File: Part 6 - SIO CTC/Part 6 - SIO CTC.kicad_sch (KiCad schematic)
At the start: 33 parts, among them J1 EDGE, J2 USB B, J3 DB9-F, J4 EXT LCD, U1 Z84C4010, U2 MCP2221A, U3 74AC138, U4 MAX232, U5 Z84C3010, U6 Z84C4010, U7 74HC563

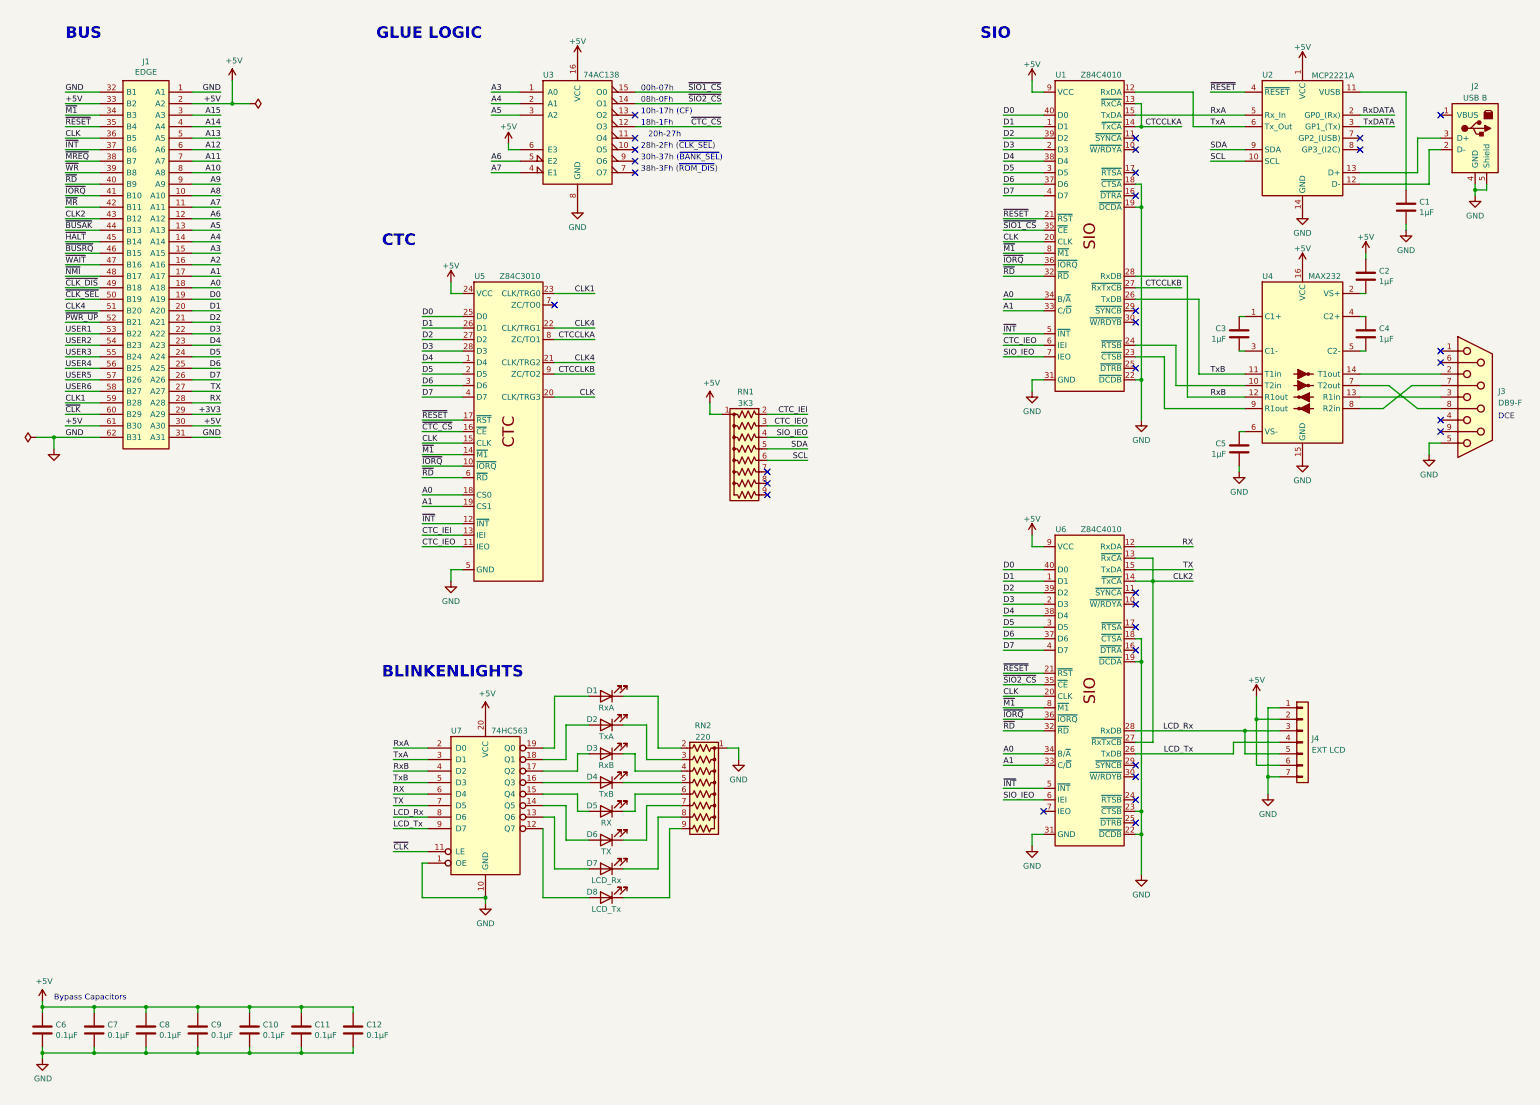
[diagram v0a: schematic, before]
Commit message: Long time backup
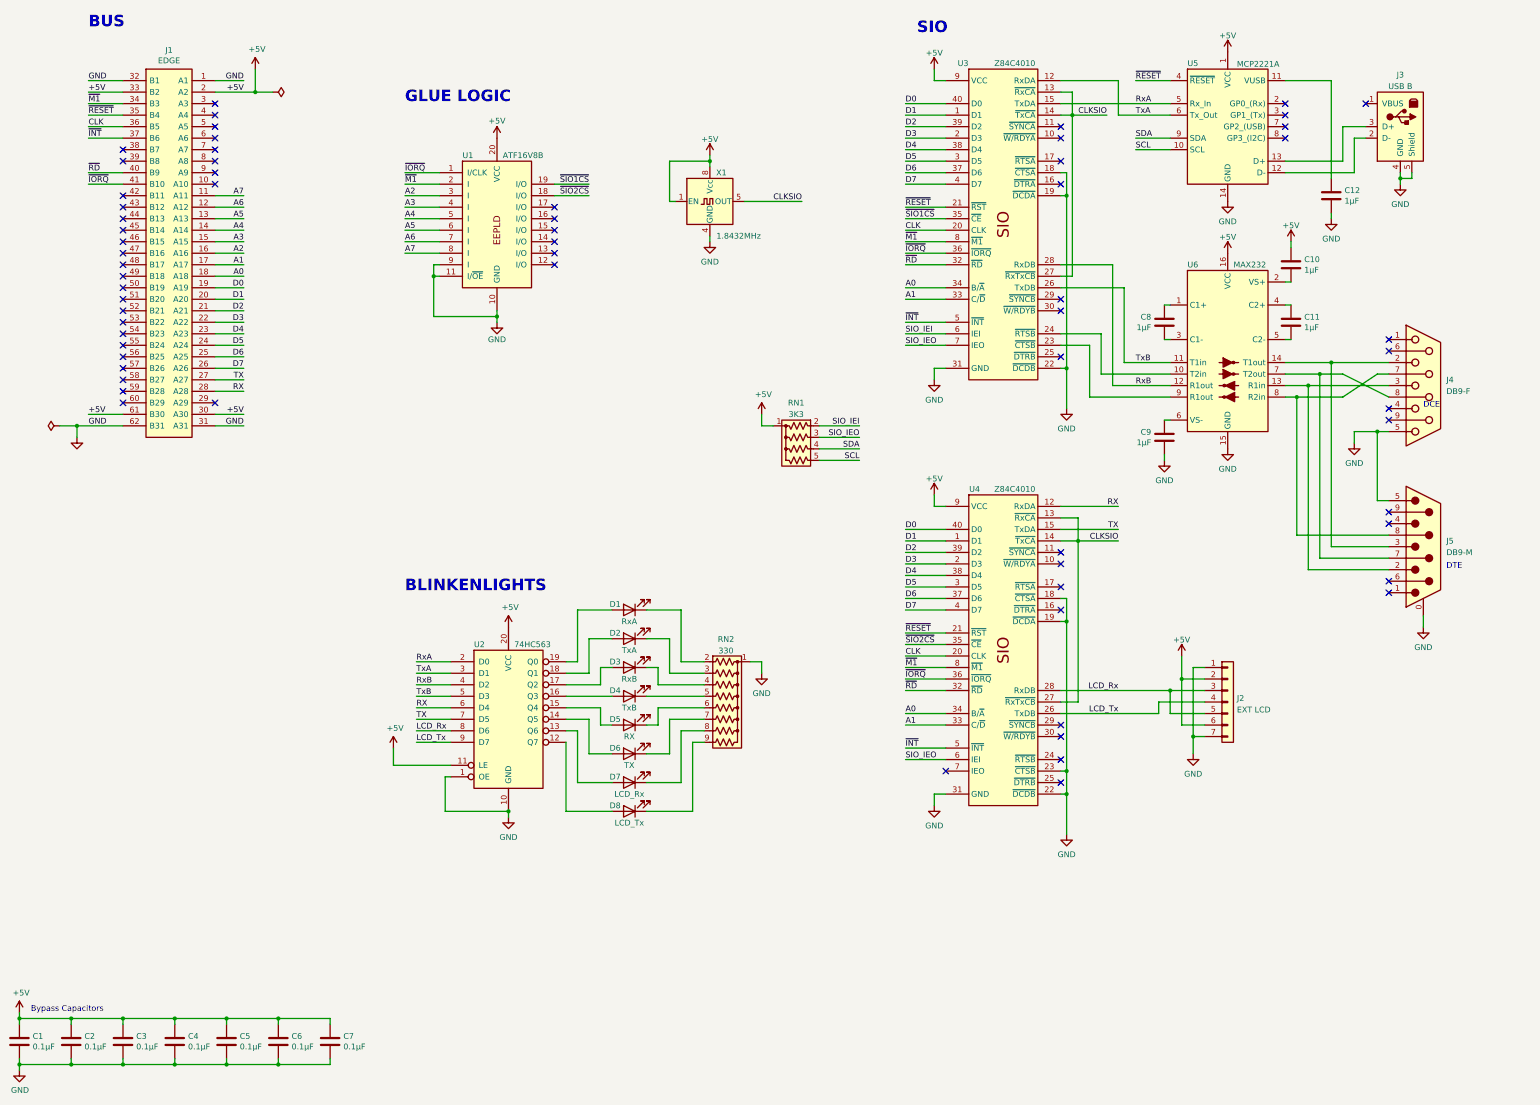
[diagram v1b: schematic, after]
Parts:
- removed RN1: 3K3, Resistor_THT:R_Array_SIP9, symbol Device:R_Network08_US
- removed U3: 74AC138, Package_DIP:DIP-16_W7.62mm_Socket, symbol 74xx:74LS138
- removed U5: Z84C3010, Package_DIP:DIP-28_W15.24mm_Socket, symbol 0_Z80_Library:Z84C30xx CTC
- added J5: DB9-M, Connector_Dsub:DSUB-9_Male_Horizontal_P2.77x2.84mm_EdgePinOffset7.70mm_Housed_MountingHolesOffset9.12mm, symbol Connector:DB9_Male_MountingHoles
- added RN1: 3K3, Resistor_THT:R_Array_SIP5, symbol Device:R_Network04_US
- added U1: ATF16V8B, Package_DIP:DIP-20_W7.62mm_Socket, symbol 0_Z80_Library:ATF16V8B
- added X1: 1.8432MHz, 0 - Library:DIP-8-4_W7.62mm_Oscillator_Socket, symbol Oscillator:CXO_DIP8
- J1: footprint 0_Z80_Library:BUS_XT -> 0 - Library:BUS_XT
- RN2: value 220 -> 330
- U3: renamed from U1; symbol 0_Z80_Library:Z84C40xx SIO -> 0_Z80_Library:Z84C40xx
- U4: renamed from U6; symbol 0_Z80_Library:Z84C40xx SIO -> 0_Z80_Library:Z84C40xx
- renumbered C6 to C1, C2 to C10, C4 to C11, C1 to C12, C7 to C2, C8 to C3, C9 to C4, C10 to C5, C11 to C6, C12 to C7, C3 to C8, C5 to C9, J4 to J2, J2 to J3, J3 to J4, U7 to U2, U2 to U5, U4 to U6
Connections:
- net CTCCLKA is gone; now on net CLKSIO: U3.13 (~{RxCA}), U3.14 (~{TxCA})
- net CTCCLKB is gone; now on net CLKSIO: U3.27 (~{RxTxCB})
- net +5V: now also U2.11 (LE), RN1.1 (common), U1.20 (VCC), X1.1 (EN), X1.8 (Vcc)
- net A2: now also U1.3 (I)
- net A3: now also U1.4 (I)
- net A4: now also U1.5 (I)
- net A5: now also U1.6 (I)
- net A6: now also U1.7 (I)
- net A7: now also U1.8 (I)
- net GND: now also J5.0 (PAD), J5.5, U1.10 (GND), U1.11 (I/~{OE}), U1.9 (I), X1.4 (GND)
- net SCL: now also RN1.5 (R4)
- net SDA: now also RN1.4 (R3)
- net SIO_IEO: now also RN1.3 (R2)
- net ~{IORQ}: now also U1.1 (I/CLK)
- net ~{M1}: now also U1.2 (I)
- net at J4.3, U6.13 (R1in): now also J5.2
- net at J4.2, U6.14 (T1out): now also J5.3
- net at J4.8, U6.7 (T2out): now also J5.7
- net at J4.7, U6.8 (R2in): now also J5.8
- net +3V3: no longer names the net of J1.29 (A29)
- net A10: no longer names the net of J1.8 (A8)
- net A11: no longer names the net of J1.7 (A7)
- net A12: no longer names the net of J1.6 (A6)
- net A13: no longer names the net of J1.5 (A5)
- net A14: no longer names the net of J1.4 (A4)
- net A15: no longer names the net of J1.3 (A3)
- net A8: no longer names the net of J1.10 (A10)
- net A9: no longer names the net of J1.9 (A9)
- net CLK1: no longer names the net of J1.59 (B28)
- net CLK2 renamed CLKSIO
- net CLKSIO: now also X1.5 (OUT); no longer J1.43 (B12)
- net CLK4: no longer names the net of J1.51 (B20)
- net CTC_IEO renamed SIO_IEI
- net SIO_IEI: now also RN1.2 (R1)
- net RxDATA: no longer names the net of U5.2 (GP0_(Rx))
- net TxDATA: no longer names the net of U5.3 (GP1_(Tx))
- net USER1: no longer names the net of J1.53 (B22)
- net USER2: no longer names the net of J1.54 (B23)
- net USER3: no longer names the net of J1.55 (B24)
- net USER4: no longer names the net of J1.56 (B25)
- net USER5: no longer names the net of J1.57 (B26)
- net USER6: no longer names the net of J1.58 (B27)
- net ~{BUSAK}: no longer names the net of J1.44 (B13)
- net ~{BUSRQ}: no longer names the net of J1.46 (B15)
- net ~{CLK_DIS}: no longer names the net of J1.49 (B18)
- net ~{CLK_SEL}: no longer names the net of J1.50 (B19)
- net ~{CLK}: no longer names the net of J1.60 (B29)
- net ~{CLK}: no longer U2.11 (LE)
- net ~{HALT}: no longer names the net of J1.45 (B14)
- net ~{MREQ}: no longer names the net of J1.38 (B7)
- net ~{MR}: no longer names the net of J1.42 (B11)
- net ~{NMI}: no longer names the net of J1.48 (B17)
- net ~{PWR_UP}: no longer names the net of J1.52 (B21)
- net ~{SIO1_CS} renamed ~{SIO1CS}
- net ~{SIO1CS}: now also U1.19 (I/O)
- net ~{SIO2_CS} renamed ~{SIO2CS}
- net ~{SIO2CS}: now also U1.18 (I/O)
- net ~{WAIT}: no longer names the net of J1.47 (B16)
- net ~{WR}: no longer names the net of J1.39 (B8)
- no-connect marks 32 -> 65
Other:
- note added: "DTE"
- note removed: "00h-07h"
- note removed: "08h-0Fh"
- note removed: "10h-17h (CF)"
- note removed: "18h-1Fh"
- note removed: "20h-27h"
- note removed: "28h-2Fh (~{CLK_SEL})"
- note removed: "30h-37h (~{BANK_SEL})"
- note removed: "38h-3Fh (~{ROM_DIS})"
- note removed: "CTC"
- moved on the sheet: C1, C10, C11, C12, C2, C3, C4, C5, C6, C7, C8, C9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
